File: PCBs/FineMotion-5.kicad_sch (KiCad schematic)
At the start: 40 parts, among them J1 Conn_01x02_Female, J2 Conn_01x04_Female, P1 USB_C_Plug_USB2.0, SW1 Option/FLASH Switch, SW3 SW_SPDT MAIN POWER, U1 ME6211C, U2 TP4056, U6 ESP-12F, U7 CH340C, U9 MPU-9250

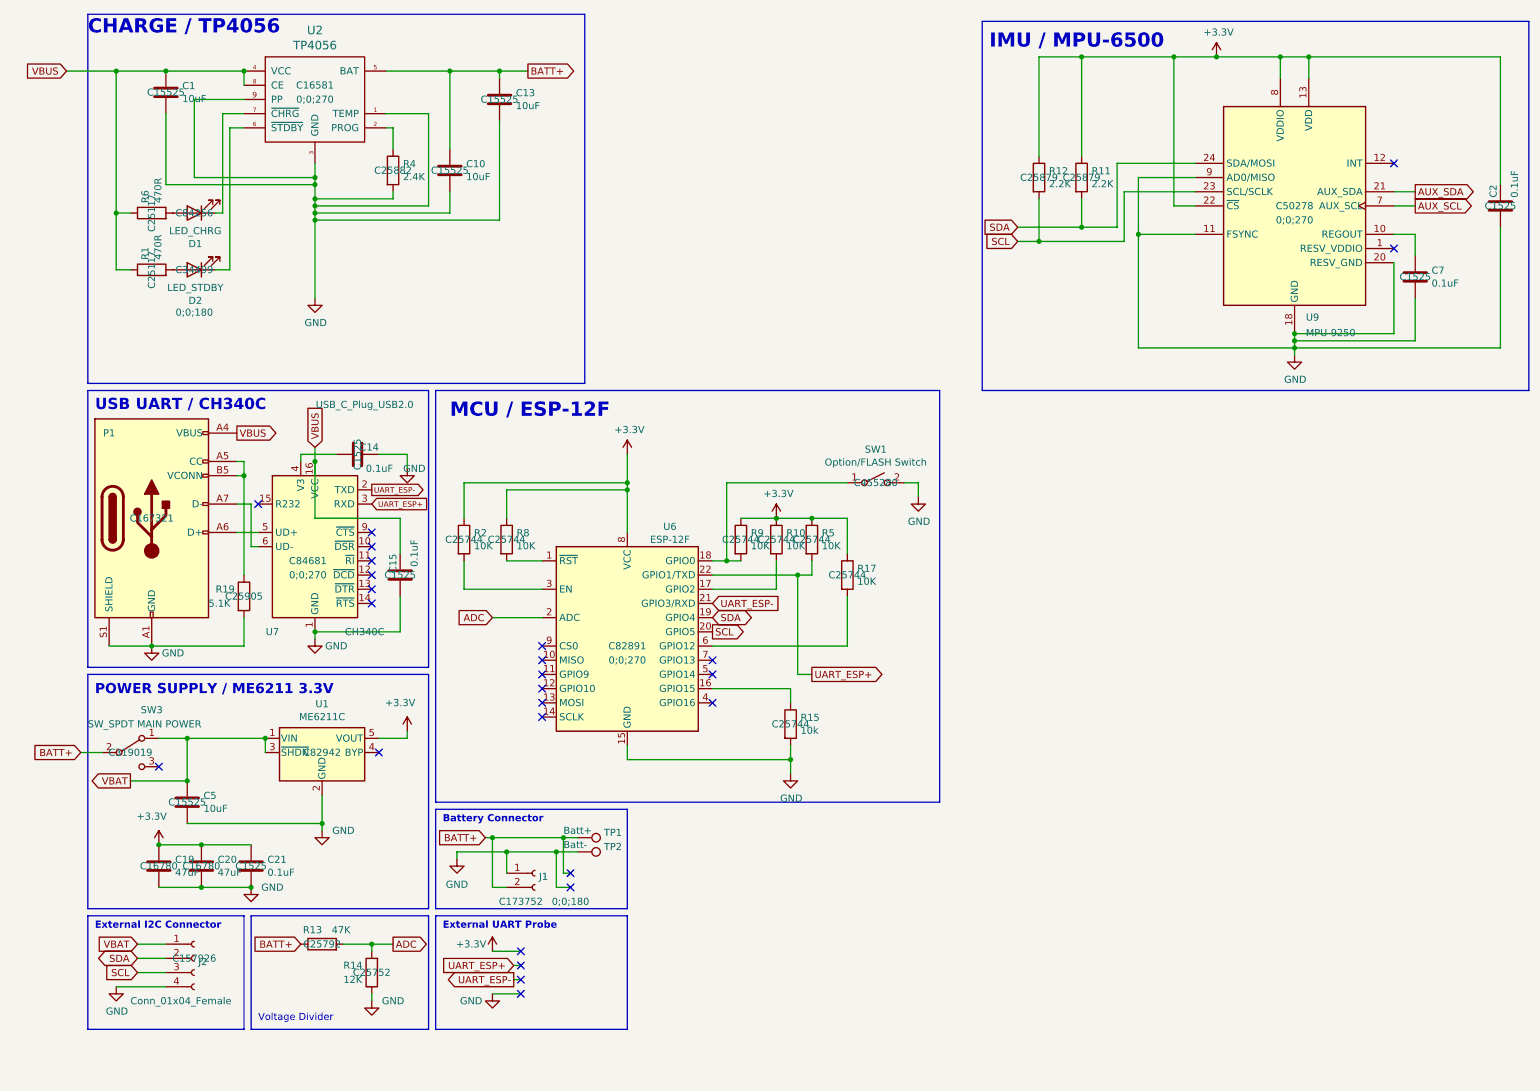
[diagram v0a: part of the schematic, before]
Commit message: bmi160
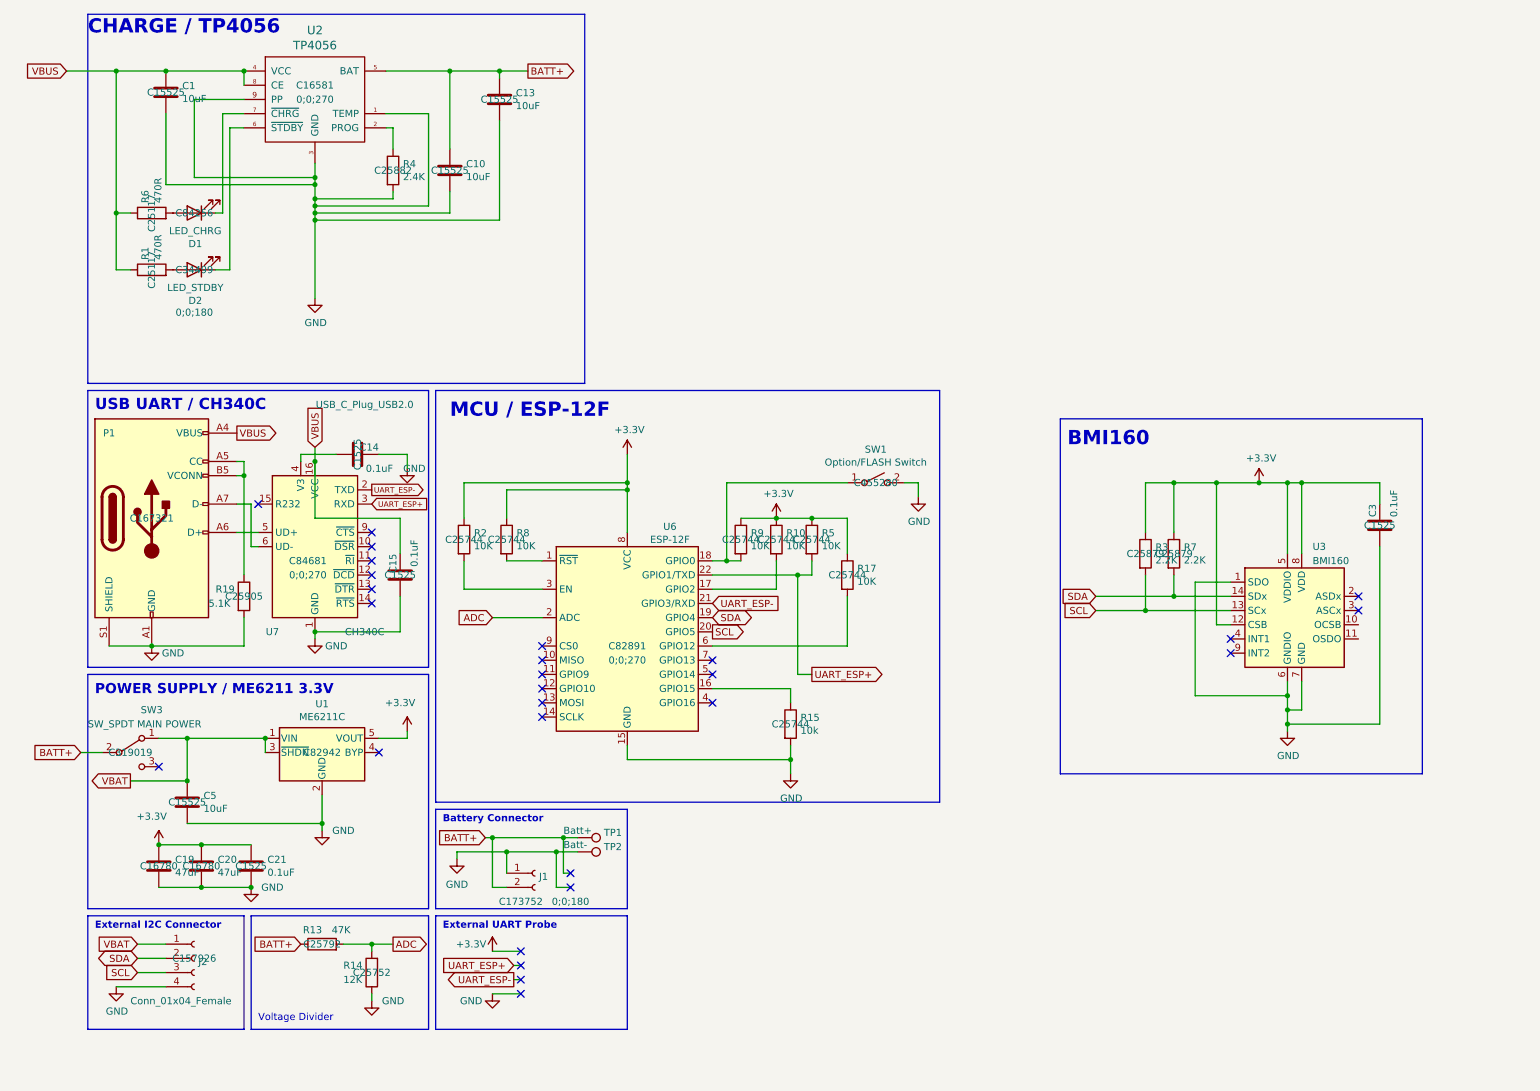
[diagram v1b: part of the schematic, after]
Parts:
- removed C2, C7: 0.1uF, Capacitor_SMD:C_0402_1005Metric, symbol Device:C
- removed R11, R12: 2.2K, Resistor_SMD:R_0402_1005Metric, symbol Device:R
- removed U9: MPU-9250, Sensor_Motion:InvenSense_QFN-24_3x3mm_P0.4mm, symbol Sensor_Motion:MPU-9250
- added C3: 0.1uF, Capacitor_SMD:C_0402_1005Metric, symbol Device:C
- added R3, R7: 2.2K, Resistor_SMD:R_0402_1005Metric, symbol Device:R
- added U3: BMI160, Package_LGA:Bosch_LGA-14_3x2.5mm_P0.5mm, symbol Sensor_Motion:BMI160
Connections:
- net +3V3: now also C3.2, R3.1, R7.1, U3.12 (CSB), U3.5 (VDDIO), U3.8 (VDD)
- net GND: now also C3.1, U3.1 (SDO), U3.6 (GNDIO), U3.7 (GND)
- net SCL: now also R3.2, U3.13 (SCx)
- net SDA: now also R7.2, U3.14 (SDx)
- no-connect marks 26 -> 28
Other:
- note added: "BMI160"
- note removed: "IMU / MPU-6500"
